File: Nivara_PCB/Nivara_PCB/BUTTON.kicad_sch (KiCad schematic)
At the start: 3 parts, among them SW1 SKRPACE010

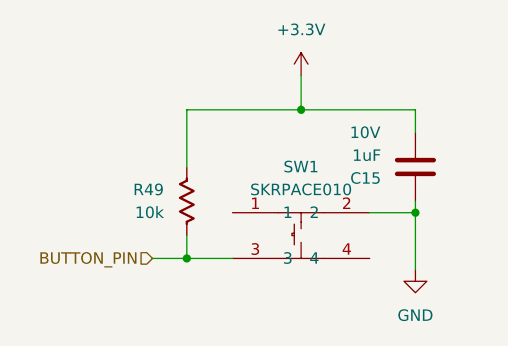
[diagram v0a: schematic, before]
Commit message: TERMINACIONES Y AJUSTES FINALES
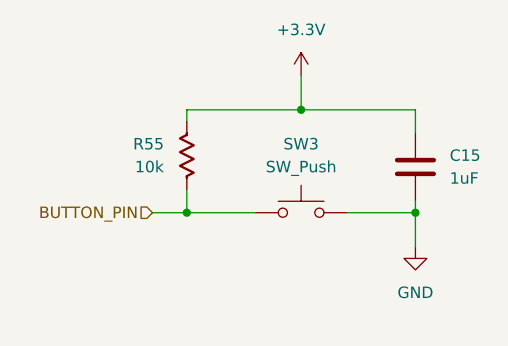
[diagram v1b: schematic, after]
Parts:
- removed SW1: SKRPACE010, EasyEDA:KEY-SMD_4P-L4.2-W3.2-P2.20-LS4.6, symbol EasyEDA:SKRPACE010
- added SW3: SW_Push, Button_Switch_SMD:SW_SPST_PTS810, symbol Switch:SW_Push
- C15: LCSC Part (none) -> C15849; Part # (none) -> CL10A105KB8NNNC; Vol 10V -> (none)
- R55: renamed from R49; LCSC Part (none) -> C25804; Part # (none) -> 0603WAF1002T5E
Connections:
- net +3.3V: now also C15.1; no longer C15.2
- net BUTTON_PIN: now also SW3.1
- net GND: now also C15.2, SW3.2; no longer C15.1
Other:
- moved on the sheet: R55
